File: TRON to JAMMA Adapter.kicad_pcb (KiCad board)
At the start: 2 copper layers, 112.2 x 98.7 mm, 58 parts, among them P1 1K, P2 10K, P3 1K, U1 74LS86, U2A 74LS191, U2B 74LS191, U3 NE555, U4 LM386, U5 NE555

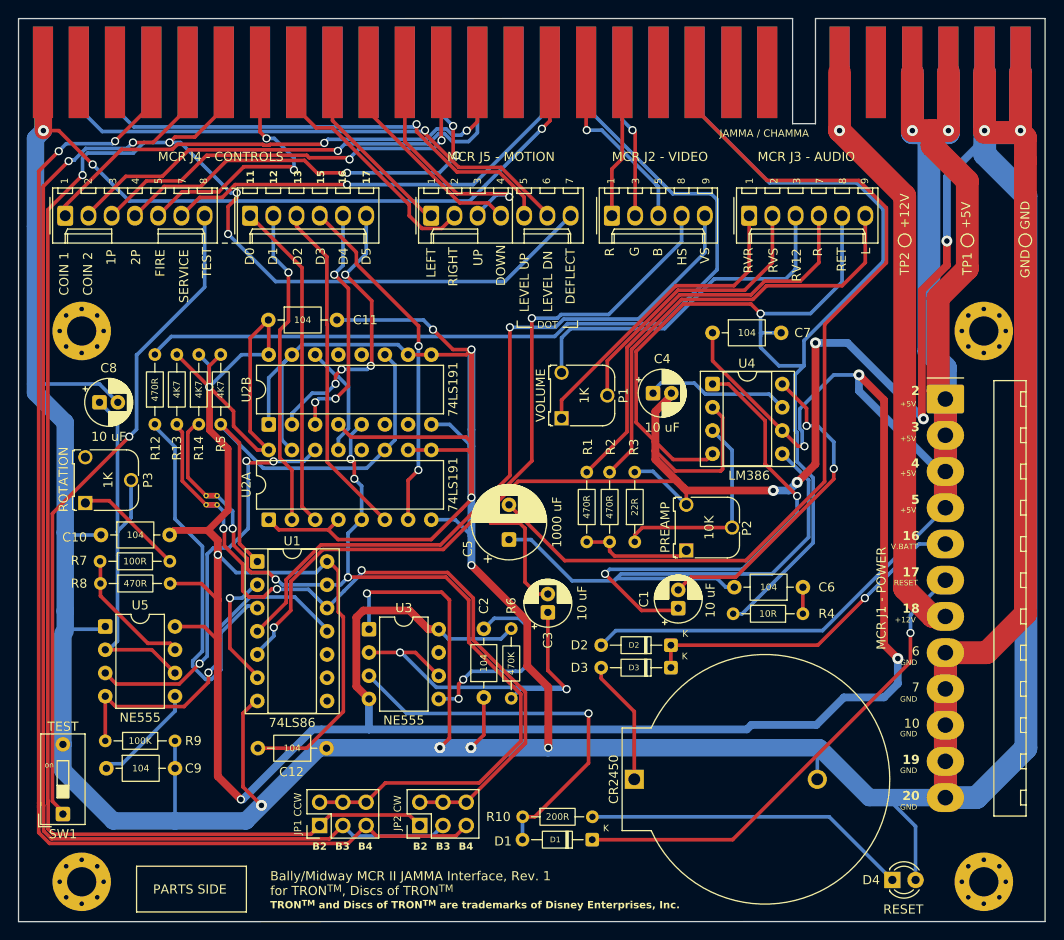
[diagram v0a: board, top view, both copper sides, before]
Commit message: miscellaneous alignment tweaks
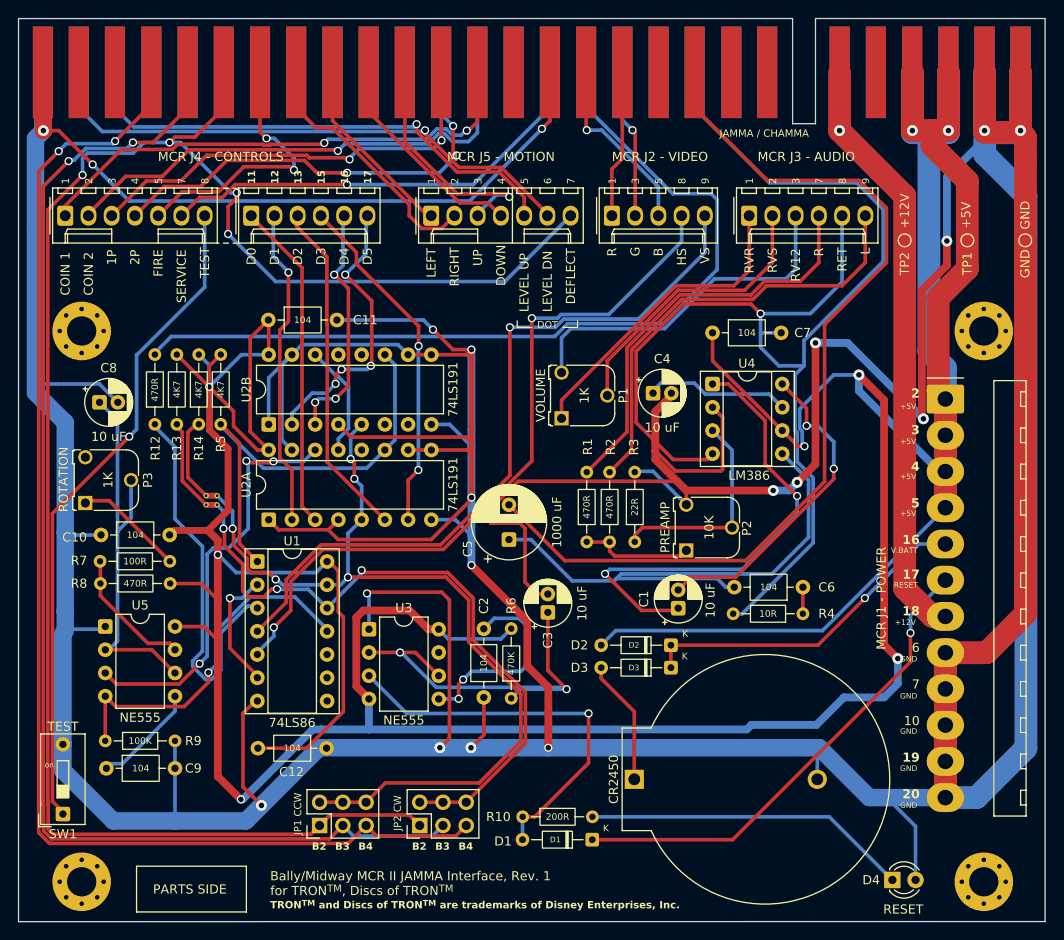
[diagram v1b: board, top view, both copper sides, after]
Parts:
- moved MCRJ4B 0.13 mm to (114.3, 66.6)
